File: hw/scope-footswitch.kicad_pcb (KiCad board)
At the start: 2 copper layers, 80 x 50 mm, 31 parts, among them J1 CN00050, J2 CN00023, J3 CN00049, SW1 M00027, SW2 M00012, SW3 M00026, Y1 Y00015

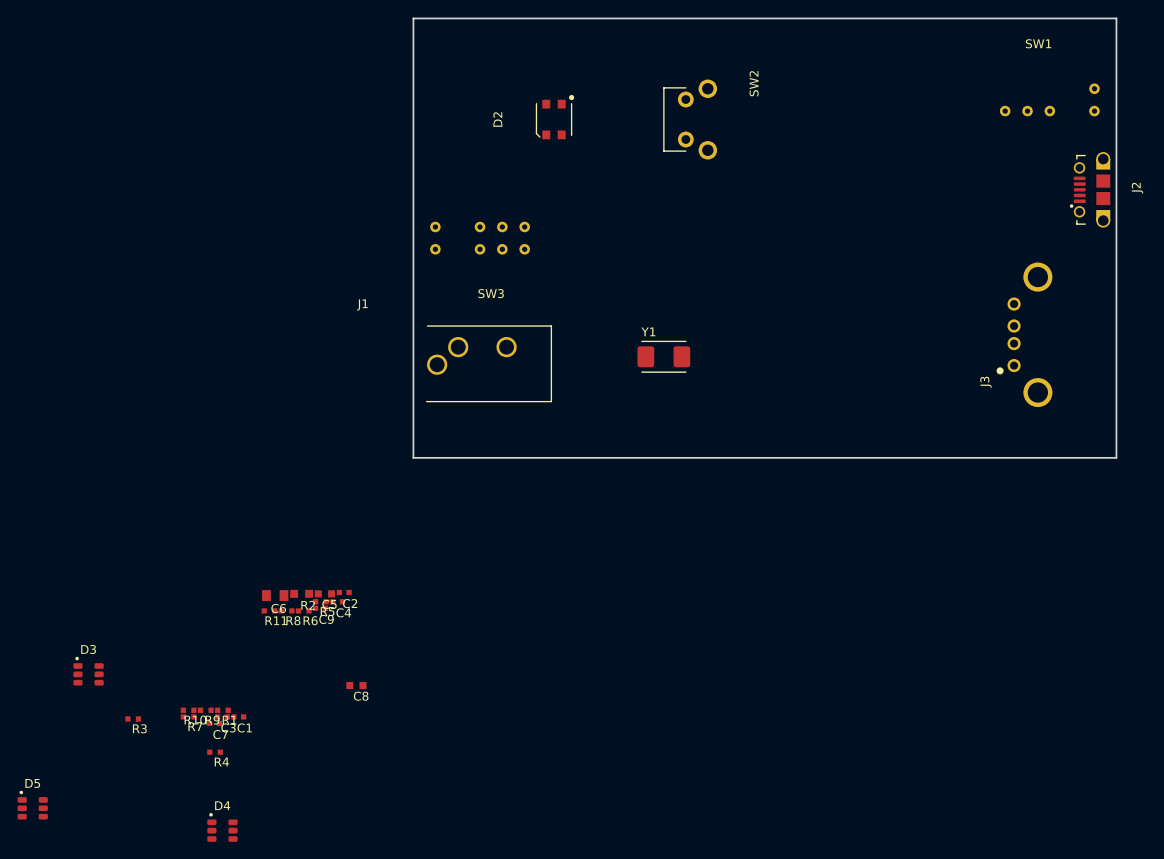
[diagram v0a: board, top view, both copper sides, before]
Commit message: Initial completion of schematic and layout
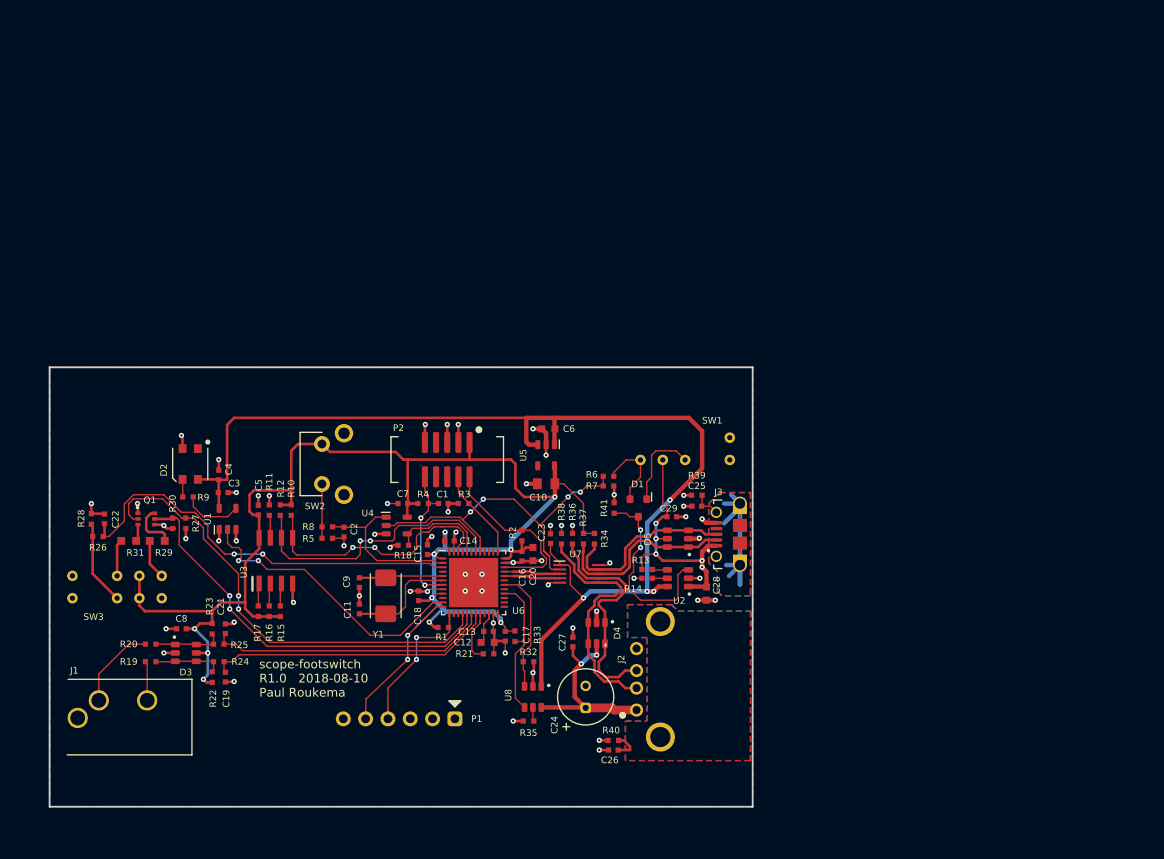
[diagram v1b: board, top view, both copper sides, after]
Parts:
- added C10: C00004, footprints:C_0805_2012M, F.Cu at (165.1, 82.5)
- added C11: C00033, footprints:C_0402_1005M, F.Cu at (143.8, 96.7)
- added C12: C00007, footprints:C_0603_1608M, F.Cu at (158.4, 100.5)
- added C13: C00001, footprints:C_0402_1005M, F.Cu at (158.6, 99.2)
- added C14: C00001, footprints:C_0402_1005M, F.Cu at (154.1, 89.0)
- added C15: C00001, footprints:C_0402_1005M, F.Cu at (151.6, 90.0)
- added C16: C00001, footprints:C_0402_1005M, F.Cu at (162.3, 90.7)
- added C17: C00001, footprints:C_0402_1005M, F.Cu at (160.4, 99.8)
- added C18: C00001, footprints:C_0402_1005M, F.Cu at (150.6, 95.2)
- added C19: C00001, footprints:C_0402_1005M, F.Cu at (128.6, 104.5)
- added C20: C00002, footprints:C_0603_1608M, F.Cu at (163.6, 90.5)
- added C21: C00001, footprints:C_0402_1005M, F.Cu at (128.6, 99.0)
- added C22: C00001, footprints:C_0402_1005M, F.Cu at (114.8, 86.5)
- added C23: C00001, footprints:C_0402_1005M, F.Cu at (165.6, 88.7)
- added C24: C00003, footprints:CRADIAL_6.3x11.2_2.5, F.Cu at (169.6, 106.7)
- added C25: C00027, footprints:C_0402_1005M, F.Cu at (182.2, 85.0)
- added C26: C00027, footprints:C_0402_1005M, F.Cu at (172.8, 112.8)
- added C27: C00001, footprints:C_0402_1005M, F.Cu at (168.2, 100.5)
- added C28: C00002, footprints:C_0603_1608M, F.Cu at (183.3, 95.0)
- added C29: C00001, footprints:C_0402_1005M, F.Cu at (179.4, 86.2)
- added D1: D00005, footprints:SOT_3_950_2900X1300X1000_ONSEMI, F.Cu at (175.6, 85.2)
- added P1: CN00052, footprints:P_FCI_68000-206, F.Cu at (148.4, 109.2)
- added P2: CN00051, footprints:P_CNC_3221-10-0300-00, F.Cu at (153.8, 79.7)
- added Q1: Q00002, footprints:SOT_6_650_2150X1300x1100_DIODES, F.Cu at (119.6, 86.5)
- added R12: R00038, footprints:R_0402_1005M, F.Cu at (134.8, 85.5)
- added R13: R00014, footprints:R_0402_1005M, F.Cu at (176.6, 92.2)
- added R14: R00009, footprints:R_0402_1005M, F.Cu at (176.6, 93.2)
- added R15: R00014, footprints:R_0402_1005M, F.Cu at (134.8, 97.0)
- added R16: R00014, footprints:R_0402_1005M, F.Cu at (133.6, 97.0)
- added R17: R00014, footprints:R_0402_1005M, F.Cu at (132.3, 97.0)
- added R18: R00014, footprints:R_0402_1005M, F.Cu at (148.8, 89.5)
- added R19: R00011, footprints:R_0402_1005M, F.Cu at (120.1, 102.7)
- added R20: R00011, footprints:R_0402_1005M, F.Cu at (120.1, 100.7)
- added R21: R00014, footprints:R_0402_1005M, F.Cu at (158.6, 101.8)
- added R22: R00014, footprints:R_0402_1005M, F.Cu at (127.1, 104.5)
- added R23: R00014, footprints:R_0402_1005M, F.Cu at (127.1, 99.0)
- added R24: R00014, footprints:R_0402_1005M, F.Cu at (127.8, 102.7)
- added R25: R00014, footprints:R_0402_1005M, F.Cu at (127.8, 100.7)
- added R26: R00014, footprints:R_0402_1005M, F.Cu at (114.1, 88.5)
- added R27: R00014, footprints:R_0402_1005M, F.Cu at (124.1, 87.0)
- added R28: R00014, footprints:R_0402_1005M, F.Cu at (113.3, 86.5)
- added R29: R00079, footprints:R_0603_1608M, F.Cu at (120.8, 89.0)
- added R30: R00014, footprints:R_0402_1005M, F.Cu at (122.6, 87.0)
- added R31: R00079, footprints:R_0603_1608M, F.Cu at (117.6, 89.0)
- added R32: R00014, footprints:R_0402_1005M, F.Cu at (163.1, 102.7)
- added R33: R00014, footprints:R_0402_1005M, F.Cu at (161.6, 99.8)
- added R34: R00047, footprints:R_0402_1005M, F.Cu at (170.6, 88.7)
- added R35: R00016, footprints:R_0402_1005M, F.Cu at (163.1, 109.5)
- added R36: R00047, footprints:R_0402_1005M, F.Cu at (168.1, 88.7)
- added R37: R00047, footprints:R_0402_1005M, F.Cu at (169.3, 88.7)
- added R38: R00047, footprints:R_0402_1005M, F.Cu at (166.8, 88.7)
- added R39: R00008, footprints:R_0402_1005M, F.Cu at (182.2, 83.8)
- added R40: R00008, footprints:R_0402_1005M, F.Cu at (172.8, 111.7)
- added R41: R00014, footprints:R_0402_1005M, F.Cu at (172.8, 85.2)
- added U1: U00054, footprints:SOT_5_950_2900X1600X1100_DIODES, F.Cu at (128.8, 86.5)
- added U2: U00086, footprints:SOT_6_950_2800x1600x110_DIODES_SOT26, F.Cu at (180.1, 93.2)
- added U3: U00055, footprints:SOIC_8_1270_4900X3900X1750, F.Cu at (134.3, 91.2)
- added U4: U00087, footprints:SOT_5_950_2900X1600X1100_DIODES, F.Cu at (148.1, 87.2)
- added U5: U00049, footprints:SOT_5_950_2900X1600X1100_DIODES, F.Cu at (165.1, 79.2)
- added U6: U00084, footprints:QFN_48_500_7000X7000X600_ST, F.Cu at (156.8, 93.7)
- added U7: U00085, footprints:MSOP_10_500_3000X3000X1100_ONSEMI, F.Cu at (168.8, 92.7)
- added U8: U00086, footprints:SOT_6_950_2800x1600x110_DIODES_SOT26, F.Cu at (163.6, 106.7)
- C2, C3: value C00033 -> C00001
- C5, C8: value C00002 -> C00001; footprint footprints:C_0603_1608M -> footprints:C_0402_1005M
- C6: value C00004 -> C00002; footprint footprints:C_0805_2012M -> footprints:C_0603_1608M
- C9: value C00001 -> C00033
- J2: value CN00023 -> CN00049; footprint footprints:J_FCI_10118194 -> footprints:J_AMPHENOL_UE27AC54100
- J3: value CN00049 -> CN00023; footprint footprints:J_AMPHENOL_UE27AC54100 -> footprints:J_FCI_10118194
- R10: value R00014 -> R00038
- R11, R4: value R00016 -> R00014
- R2: value R00025 -> R00016; footprint R_0603_1608M -> footprints:R_0402_1005M
- R7: value R00014 -> R00056
- R9: value R00009 -> R00037
- moved D5 79.6 mm to (180.1, 88.7), turned to 180 degrees
- moved J2 75.1 mm to (178.1, 104.7)
- moved SW1 57.4 mm to (186.0, 78.5)
- moved J1 57.3 mm to (110.6, 108.2)
- moved SW3 57.3 mm to (111.2, 94.2)
- moved D2 57.0 mm to (124.6, 80.2)
- moved SW2 57.0 mm to (139.6, 80.2)
- moved R7 54.5 mm to (172.2, 82.7), turned to 180 degrees
- moved D4 48.1 mm to (170.8, 99.5), turned to 270 degrees
- moved R3 44.9 mm to (155.7, 84.7), turned to 180 degrees
- moved Y1 41.7 mm to (146.8, 95.2), turned to 270 degrees
- moved J3 40.8 mm to (187.2, 88.2)
- moved R6 37.9 mm to (172.2, 81.6)
- moved R4 36.9 mm to (151.1, 84.7)
- moved C6 36.4 mm to (165.3, 76.2)
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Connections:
- C2 pad 1: GND -> /BTN
- C2 pad 2: Net-(C2-Pad2) -> GND
- C3 pad 1: GND -> +5V
- C3 pad 2: Net-(C3-Pad2) -> GND
- C4 pad 1: /BTN -> +5V
- C5 pad 1: GND -> +3V3
- C5 pad 2: +5V -> GND
- C6 pad 1: +3V3 -> GND
- C6 pad 2: GND -> +5V
- C7 pad 1: /HOST_VBUS -> +3V3
- C8 pad 1: GND -> +3V3
- C8 pad 2: VBUS -> GND
- C9 pad 1: VBUS -> GND
- C9 pad 2: GND -> Net-(C9-Pad2)
- D2 pad 2: Net-(D2-Pad2) -> GND
- D2 pad 3: (no net) -> /LED_DATA
- D2 pad 4: Net-(D2-Pad4) -> +5V
- D3 pad 1: Net-(D3-Pad1) -> /FOOTSW_BTN1_R
- D3 pad 2: Net-(D3-Pad2) -> GND
- D3 pad 3: Net-(D3-Pad3) -> /FOOTSW_BTN2_R
- D3 pad 4: Net-(D3-Pad4) -> /FOOTSW_BTN2_R
- D3 pad 5: Net-(D3-Pad5) -> +3V3
- D3 pad 6: Net-(D3-Pad6) -> /FOOTSW_BTN1_R
- D4 pad 1: Net-(D4-Pad1) -> /HOST_DP
- D4 pad 3: GND -> /HOST_DM
- D4 pad 4: GND -> /HOST_DM
- D4 pad 5: VBUS -> /HOST_VBUS
- D4 pad 6: Net-(D4-Pad6) -> /HOST_DP
- D5 pad 1: Net-(D5-Pad1) -> /DEVICE_DM
- D5 pad 3: Net-(D5-Pad3) -> /DEVICE_DP
- D5 pad 4: Net-(D5-Pad4) -> /DEVICE_DP
- D5 pad 5: /HOST_VBUS -> VBUS
- D5 pad 6: Net-(D5-Pad6) -> /DEVICE_DM
- J1 pad 1: Net-(J1-Pad1) -> GND
- J2 pad 1: VBUS -> /HOST_VBUS
- J2 pad 2: Net-(D4-Pad1) -> /HOST_DM
- J2 pad 3: Net-(D4-Pad6) -> /HOST_DP
- J2 pad 4: Net-(J2-Pad4) -> GND
- J2 pad M1: Net-(J2-PadM1) -> /HOST_SHIELD
- J2 pad M2: Net-(J2-PadM1) -> /HOST_SHIELD
- J3 pad 1: /HOST_VBUS -> VBUS
- J3 pad 2: Net-(D5-Pad1) -> /DEVICE_DM
- J3 pad 3: Net-(D5-Pad6) -> /DEVICE_DP
- J3 pad 4: GND -> Net-(J3-Pad4)
- J3 pad M1: Net-(J3-PadM1) -> /DEVICE_SHIELD
- J3 pad M2: Net-(J3-PadM2) -> /DEVICE_SHIELD
- R1 pad 1: /EN_DEVICE -> +3V3
- R1 pad 2: /EN_DEVICE_5V -> /UART_RX
- R10 pad 1: +3V3 -> /I2C_SDA
- R10 pad 2: /HOST_FAULT_N -> +3V3
- R11 pad 1: /HOST_ILIM -> GND
- R11 pad 2: GND -> Net-(R11-Pad2)
- R2 pad 1: /EN_DEVICE -> +3V3
- R2 pad 2: GND -> /SWDIO
- R3 pad 1: +3V3 -> /SWDCLK
- R3 pad 2: /SWDIO -> GND
- R4 pad 1: /SWDCLK -> +3V3
- R4 pad 2: GND -> /NRST
- R5 pad 1: /NRST -> /BTN_R
- R5 pad 2: +3V3 -> GND
- R6 pad 1: /BTN_R -> /EN_DEVICE
- R6 pad 2: /BTN -> /EN_DEVICE_5V
- R7 pad 1: /BTN -> GND
- R7 pad 2: GND -> /EN_DEVICE
- R8 pad 1: VBUS -> /BTN_R
- R8 pad 2: /VIN_FAULT_N -> /BTN
- R9 pad 1: /VIN_ILIM -> /LED_DATA
- R9 pad 2: GND -> /LED_DATA_R
- SW3 pad 2: Net-(SW3-Pad2) -> +3V3
- SW3 pad 3: Net-(SW3-Pad3) -> /MODE_R
- SW3 pad 5: Net-(SW3-Pad5) -> +3V3
- Y1 pad 1: Net-(C2-Pad2) -> Net-(C9-Pad2)
- Y1 pad 2: Net-(C3-Pad2) -> Net-(C11-Pad2)
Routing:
- net +3V3: track 0.00 -> 171.1 mm, vias 0 -> 10
- net +5V: track 0.00 -> 127.2 mm, vias 0 -> 4
- net GND: track 0.00 -> 100.7 mm, vias 0 -> 61
- net /MODE_LED_R: track 0.00 -> 53.1 mm, vias 0 -> 2
- net /MODE: track 0.00 -> 47.3 mm, vias 0 -> 2
- net /MODE_LED_G: track 0.00 -> 46.7 mm, vias 0 -> 2
- net /EN_DEVICE: track 0.00 -> 42.9 mm, vias 0 -> 4
- net /LED_DATA_LS: track 0.00 -> 33.1 mm, vias 0 -> 2
- net /FOOTSW_BTN2: track 0.00 -> 32.9 mm
- net /I2C_SCL: track 0.00 -> 32.6 mm, vias 0 -> 2
- net /FOOTSW_BTN1: track 0.00 -> 32.2 mm
- net VBUS: track 0.00 -> 29.9 mm, vias 0 -> 5
- net /I2C_SDA: track 0.00 -> 29.3 mm, vias 0 -> 2
- net /HOST_DM: track 0.00 -> 27.9 mm
- net /HOST_DP: track 0.00 -> 26.9 mm
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- added copper zone on B.Cu, net /DEVICE_SHIELD
- added copper zone on F.Cu, net /DEVICE_SHIELD
- added copper zone on B.Cu, net /HOST_SHIELD
- added copper zone on F.Cu, net /HOST_SHIELD
- added copper zone on B.Cu, net GND
- added copper zone on F.Cu, net GND
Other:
- net class Default: clearance 0.2 -> 0.16; trace_width 0.25 -> 0.16; via_dia 0.8 -> 0.6; via_drill 0.4 -> 0.26
- net class POWER added: clearance 0.16, trace_width 0.3, via_dia 0.6, via_drill 0.26
- net class USB added: clearance 0.16, trace_width 0.3, via_dia 0.6, via_drill 0.26
- rule pad_to_mask_clearance: 0.2 -> 0.0508
- rule trace_clearance: 0.2 -> 0.16
- rule trace_min: 0.2 -> 0.16
- rule via_min_drill: 0.3 -> 0.26
- rule via_min_size: 0.4 -> 0.6
- board text added: "scope-footswitch R1.0 2018-08-10 Paul Roukema"
